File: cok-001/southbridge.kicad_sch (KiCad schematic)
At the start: 8 parts, among them U3001 CXD2973GB

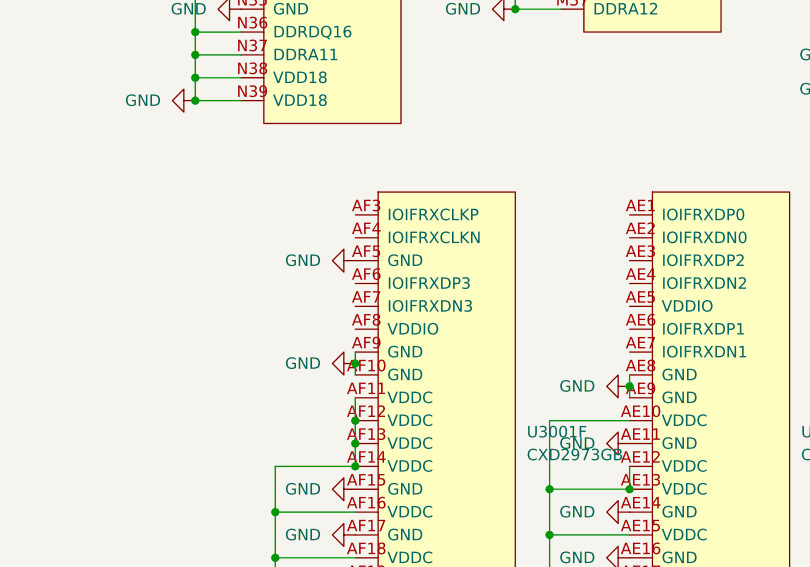
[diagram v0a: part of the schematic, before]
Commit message: rdy
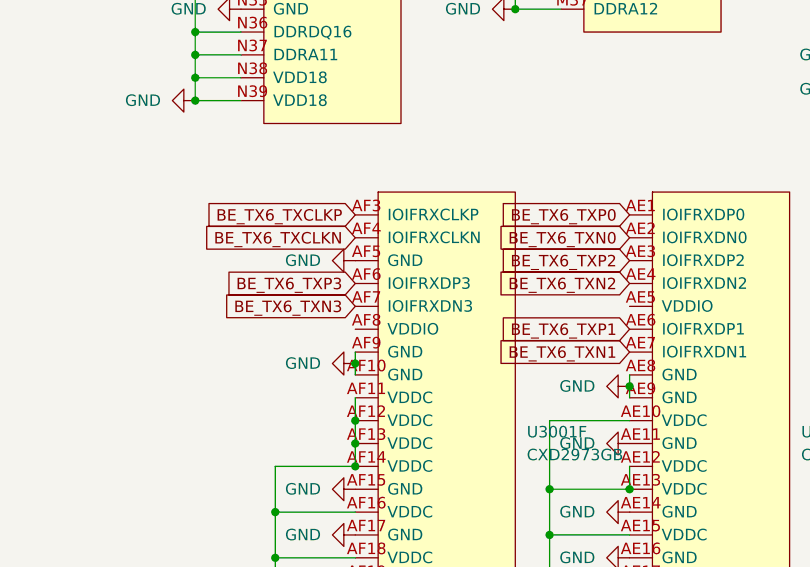
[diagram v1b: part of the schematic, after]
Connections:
- net BE_TX6_TXCLKP: now reaches U3001.AF3 (IOIFRXCLKP)
- net BE_TX6_TXCLKN: now reaches U3001.AF4 (IOIFRXCLKN)
- net BE_TX6_TXP3: now reaches U3001.AF6 (IOIFRXDP3)
- net BE_TX6_TXN3: now reaches U3001.AF7 (IOIFRXDN3)
- net BE_TX6_TXP0: now reaches U3001.AE1 (IOIFRXDP0)
- net BE_TX6_TXN0: now reaches U3001.AE2 (IOIFRXDN0)
- net BE_TX6_TXP2: now reaches U3001.AE3 (IOIFRXDP2)
- net BE_TX6_TXN2: now reaches U3001.AE4 (IOIFRXDN2)
- net BE_TX6_TXP1: now reaches U3001.AE6 (IOIFRXDP1)
- net BE_TX6_TXN1: now reaches U3001.AE7 (IOIFRXDN1)
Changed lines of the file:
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@@
 		)
 	)
+	(global_label "BE_TX6_TXN1"
+		(shape input)
+		(at 119.38 166.37 180)
+		(fields_autoplaced yes)
+		(effects
+			(font
+				(size 1.27 1.27)
+			)
+			(justify right)
+		)
+		(property "Intersheetrefs" "${INTERSHEET_REFS}"
+			(at 103.9369 166.37 0)
+			(effects
+				(font
+					(size 1.27 1.27)
+				)
+				(justify right)
+				(hide yes)
+			)
+		)
+	)
 	(global_label "SB_PEX_AMOUT"
 		(shape output)
@@
 		)
 	)
+	(global_label "BE_TX6_TXN0"
+		(shape input)
+		(at 119.38 153.67 180)
+		(fields_autoplaced yes)
+		(effects
+			(font
+				(size 1.27 1.27)
+			)
+			(justify right)
+		)
+		(property "Intersheetrefs" "${INTERSHEET_REFS}"
+			(at 103.9369 153.67 0)
+			(effects
+				(font
+					(size 1.27 1.27)
+				)
+				(justify right)
+				(hide yes)
+			)
+		)
+	)
 	(global_label "SB_PCIHOST"
 		(shape input)
@@
 		)
 	)
+	(global_label "BE_TX6_TXN3"
+		(shape input)
+		(at 88.9 161.29 180)
+		(fields_autoplaced yes)
+		(effects
+			(font
+				(size 1.27 1.27)
+			)
+			(justify right)
+		)
+		(property "Intersheetrefs" "${INTERSHEET_REFS}"
+			(at 73.4569 161.29 0)
+			(effects
+				(font
+					(size 1.27 1.27)
+				)
+				(justify right)
+				(hide yes)
+			)
+		)
+	)
 	(global_label "BE_TX6_TXP7"
 		(shape input)
@@
 		)
 	)
+	(global_label "BE_TX6_TXP1"
+		(shape input)
+		(at 119.38 163.83 180)
+		(fields_autoplaced yes)
+		(effects
+			(font
+				(size 1.27 1.27)
+			)
+			(justify right)
+		)
+		(property "Intersheetrefs" "${INTERSHEET_REFS}"
+			(at 103.9974 163.83 0)
+			(effects
+				(font
+					(size 1.27 1.27)
+				)
+				(justify right)
+				(hide yes)
+			)
+		)
+	)
 	(global_label "SB_PCI_AD13_SB"
 		(shape bidirectional)
@@
 		)
 	)
+	(global_label "BE_TX6_TXCLKP"
+		(shape input)
+		(at 88.9 151.13 180)
+		(fields_autoplaced yes)
+		(effects
+			(font
+				(size 1.27 1.27)
+			)
+			(justify right)
+		)
+		(property "Intersheetrefs" "${INTERSHEET_REFS}"
+			(at 71.1588 151.13 0)
+			(effects
+				(font
+					(size 1.27 1.27)
+				)
+				(justify right)
+				(hide yes)
+			)
+		)
+	)
 	(global_label "~{SB_ATA0_DIOW}"
 		(shape output)
@@
 		)
 	)
+	(global_label "BE_TX6_TXP2"
+		(shape input)
+		(at 119.38 156.21 180)
+		(fields_autoplaced yes)
+		(effects
+			(font
+				(size 1.27 1.27)
+			)
+			(justify right)
+		)
+		(property "Intersheetrefs" "${INTERSHEET_REFS}"
+			(at 103.9974 156.21 0)
+			(effects
+				(font
+					(size 1.27 1.27)
+				)
+				(justify right)
+				(hide yes)
+			)
+		)
+	)
 	(global_label "~{SB_RESET}"
 		(shape input)
@@
 		)
 	)
+	(global_label "BE_TX6_TXP3"
+		(shape input)
+		(at 88.9 158.75 180)
+		(fields_autoplaced yes)
+		(effects
+			(font
+				(size 1.27 1.27)
+			)
+			(justify right)
+		)
+		(property "Intersheetrefs" "${INTERSHEET_REFS}"
+			(at 73.5174 158.75 0)
+			(effects
+				(font
+					(size 1.27 1.27)
+				)
+				(justify right)
+				(hide yes)
+			)
+		)
+	)
 	(global_label "SB_PCI_AD24_SB"
 		(shape bidirectional)
@@
 		)
 	)
+	(global_label "BE_TX6_TXN2"
+		(shape input)
+		(at 119.38 158.75 180)
+		(fields_autoplaced yes)
+		(effects
+			(font
+				(size 1.27 1.27)
+			)
+			(justify right)
+		)
+		(property "Intersheetrefs" "${INTERSHEET_REFS}"
+			(at 103.9369 158.75 0)
+			(effects
+				(font
+					(size 1.27 1.27)
+				)
+				(justify right)
+				(hide yes)
+			)
+		)
+	)
 	(global_label "SB_GBE_TXD7"
 		(shape output)
@@
 		)
 	)
+	(global_label "BE_TX6_TXCLKN"
+		(shape input)
+		(at 88.9 153.67 180)
+		(fields_autoplaced yes)
+		(effects
+			(font
+				(size 1.27 1.27)
+			)
+			(justify right)
+		)
+		(property "Intersheetrefs" "${INTERSHEET_REFS}"
+			(at 71.0983 153.67 0)
+			(effects
+				(font
+					(size 1.27 1.27)
+				)
+				(justify right)
+				(hide yes)
+			)
+		)
+	)
 	(global_label "SB_ATA0_DD12"
 		(shape output)
@@
 			(effects
 				(font
+					(size 1.27 1.27)
+				)
+				(justify right)
+				(hide yes)
+			)
+		)
+	)
+	(global_label "BE_TX6_TXP0"
+		(shape input)
+		(at 119.38 151.13 180)
+		(fields_autoplaced yes)
+		(effects
+			(font
+				(size 1.27 1.27)
+			)
+			(justify right)
+		)
+		(property "Intersheetrefs" "${INTERSHEET_REFS}"
+			(at 103.9974 151.13 0)
+			(effects
+				(font
